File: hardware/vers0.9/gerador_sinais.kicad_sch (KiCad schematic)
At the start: 6 parts, among them J1 Conn_02x03_Odd_Even, J2 Conn_02x05_Odd_Even, J3 Conn_01x03, U2 74HC138

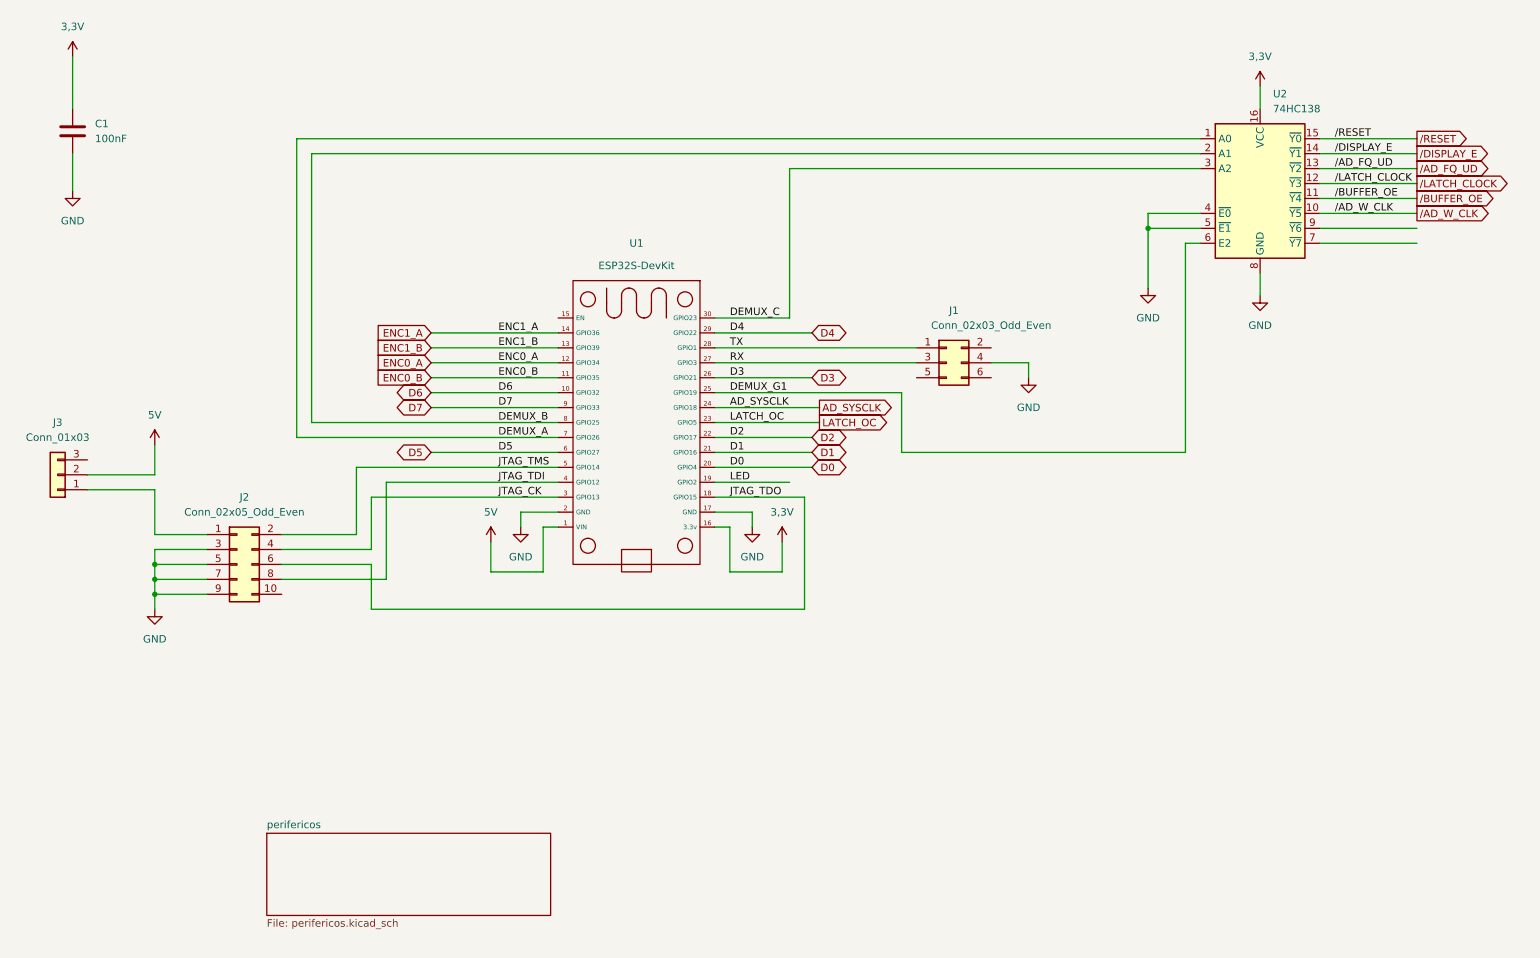
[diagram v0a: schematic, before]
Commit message: 250330-0836
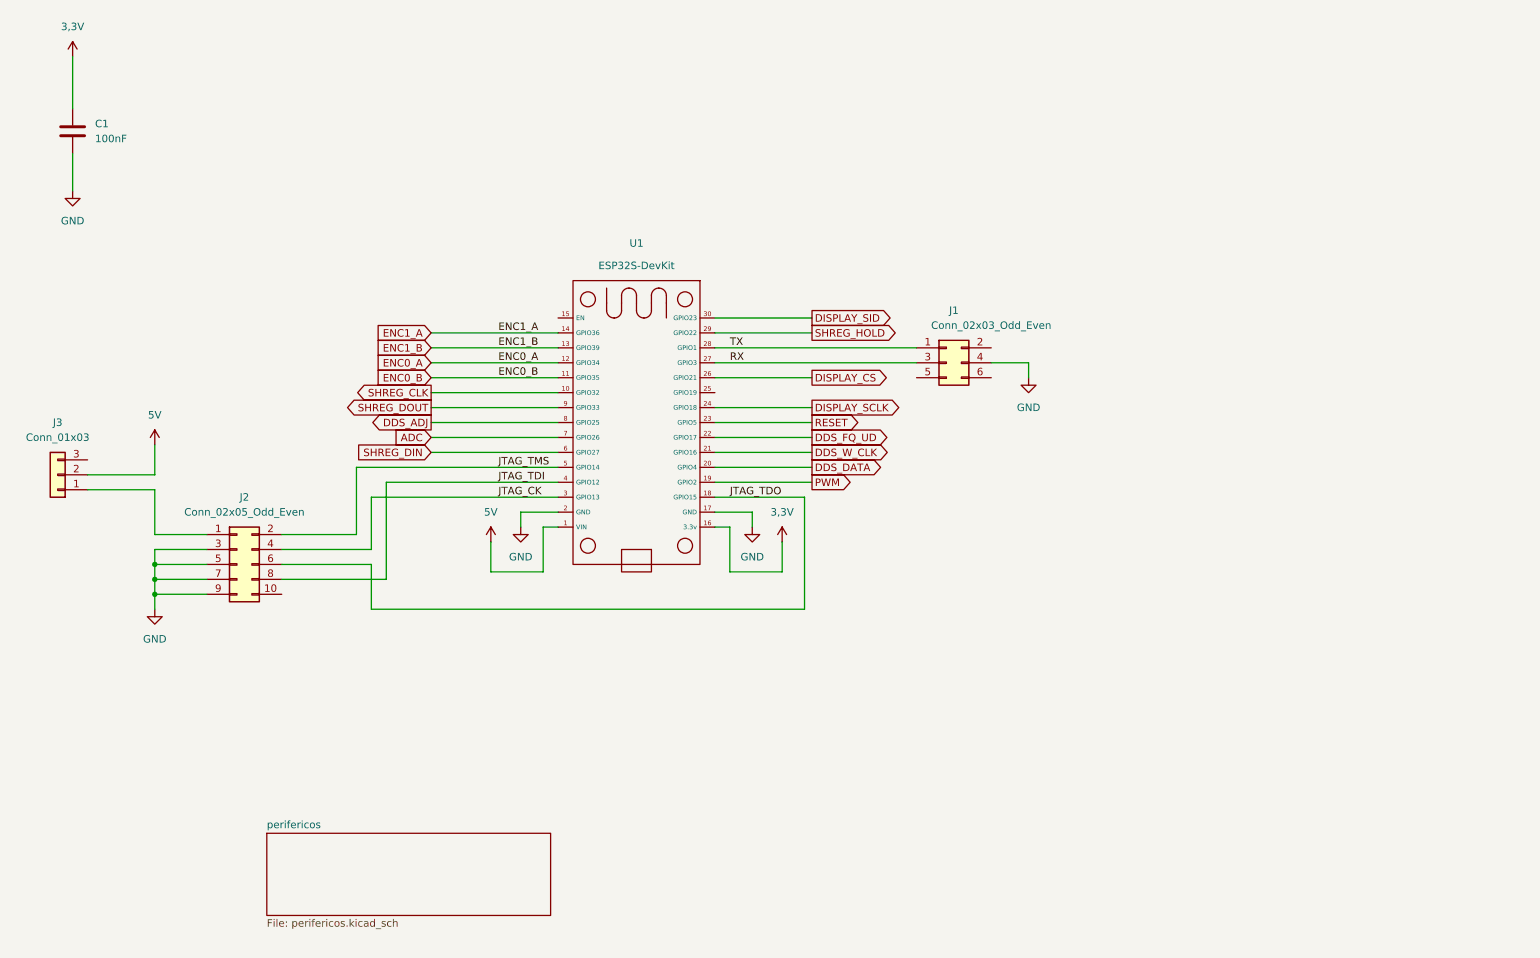
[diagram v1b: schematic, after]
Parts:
- removed U2: 74HC138, symbol 74xx:74HC138
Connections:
- net AD_SYSCLK renamed DISPLAY_SCLK
- net D0 renamed DDS_DATA
- net D1 renamed DDS_W_CLK
- net D2 renamed DDS_FQ_UD
- net D3 renamed DISPLAY_CS
- net D4 renamed SHREG_HOLD
- net D5 renamed SHREG_DIN
- net D6 renamed SHREG_CLK
- net D7 renamed SHREG_DOUT
- net DEMUX_A renamed ADC
- net DEMUX_B renamed DDS_ADJ
- net DEMUX_C renamed DISPLAY_SID
- net DEMUX_G1: no longer names the net of U1.25 (GPIO19)
- net LATCH_OC renamed RESET
- net LED renamed PWM

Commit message: 250404-0705
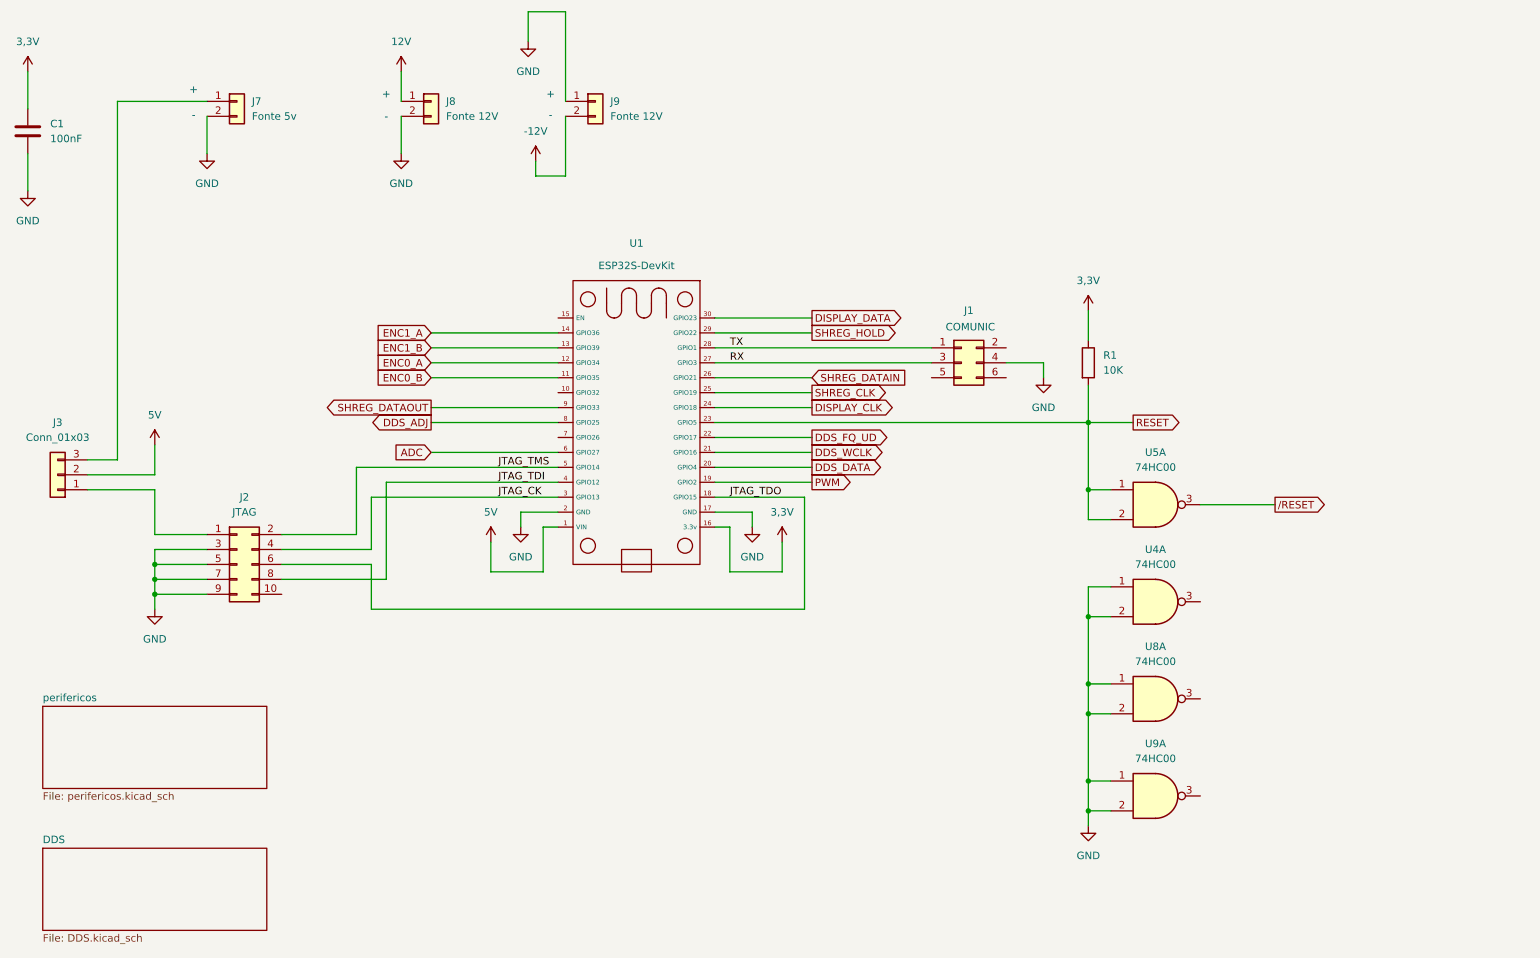
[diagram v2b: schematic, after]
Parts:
- added J7: Fonte 5v, symbol Connector_Generic:Conn_01x02
- added J8, J9: Fonte 12V, symbol Connector_Generic:Conn_01x02
- added R1: 10K, symbol Device:R
- added U4, U5, U8, U9: 74HC00, symbol 74xx:74HC00
- J1: value Conn_02x03_Odd_Even -> COMUNIC
- J2: value Conn_02x05_Odd_Even -> JTAG
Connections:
- net SHREG_DIN is gone; now on net ADC: U1.6 (GPIO27)
- net 3,3V: now also R1.1
- net ADC: no longer U1.7 (GPIO26)
- net GND: now also J7.2 (Pin_2), J8.2 (Pin_2), J9.1 (Pin_1), U4.1, U4.2, U8.1, U8.2, U9.1, U9.2
- net RESET: now also R1.2, U5.1, U5.2
- net SHREG_CLK: now also U1.25 (GPIO19); no longer U1.10 (GPIO32)
- net at J3.3 (Pin_3): now also J7.1 (Pin_1)
- net DDS_W_CLK renamed DDS_WCLK
- net DISPLAY_CS renamed SHREG_DATAIN
- net DISPLAY_SCLK renamed DISPLAY_CLK
- net DISPLAY_SID renamed DISPLAY_DATA
- net SHREG_DOUT renamed SHREG_DATAOUT
- new net -12V: J9.2 (Pin_2)
- new net 12V: J8.1 (Pin_1)
- new net /RESET: U5.3
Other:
- added sheet DDS (DDS.kicad_sch)
- note added: "+"
- note added: "-"
- moved on the sheet: C1, J1

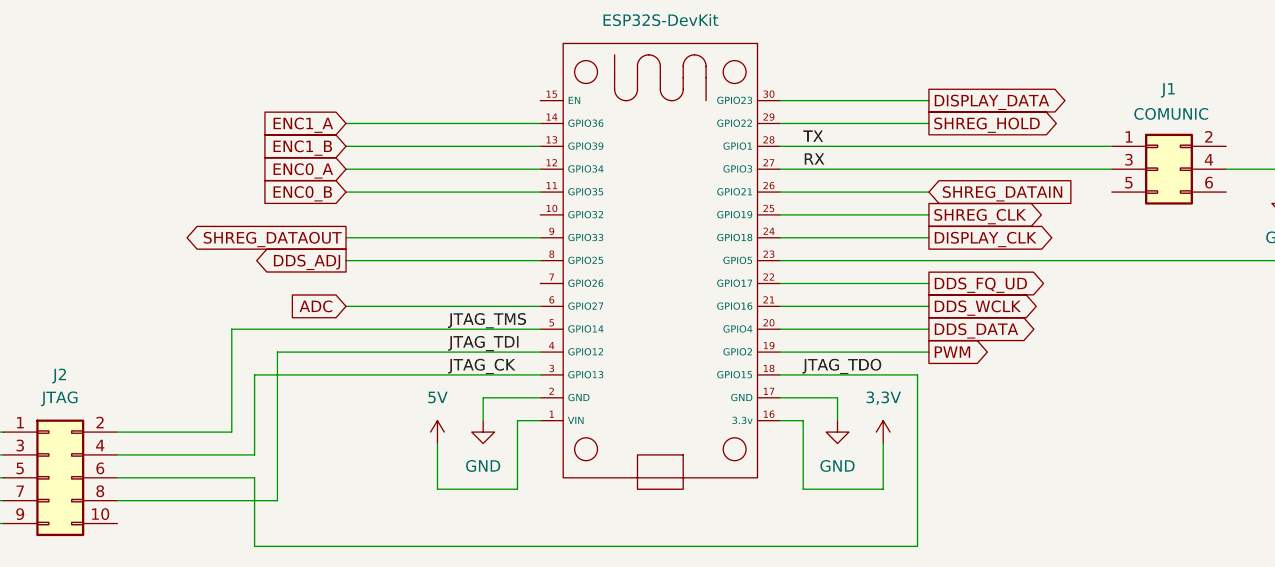
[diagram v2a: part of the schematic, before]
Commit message: 250425-1655
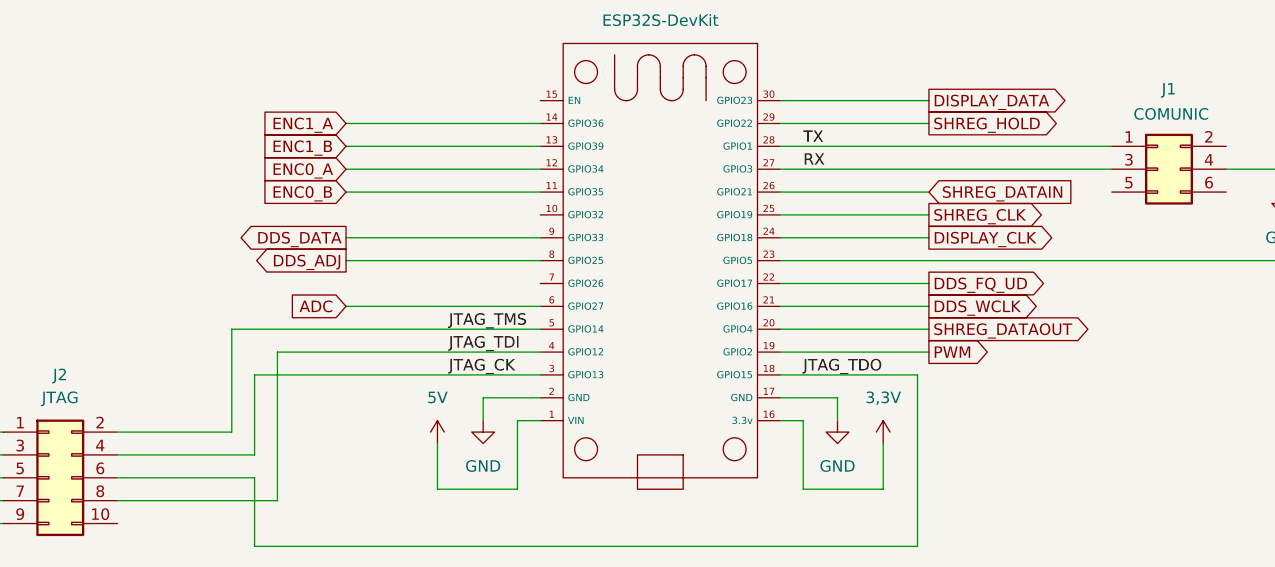
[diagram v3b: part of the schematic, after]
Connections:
- net DDS_DATA: now also U1.9 (GPIO33); no longer U1.20 (GPIO4)
- net SHREG_DATAOUT: now also U1.20 (GPIO4); no longer U1.9 (GPIO33)
